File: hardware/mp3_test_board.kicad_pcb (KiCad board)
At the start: 4 copper layers, 99.5 x 56 mm, 224 parts, among them J1 TF01-A, J2 PJ-322, P1 WF24LTYAJDNN0#, P2 USB-TYPE-C-018, Q1 2N7002K, SW1 K2-1156SP-F5SW-05, SW2 K2-1156SP-F5SW-05, SW3 K2-1156SP-F5SW-05, SW4 K2-1156SP-F5SW-05, SW5 K2-1156SP-F5SW-05, SW6 GT-TC054A-H035-L1, SW7 GT-TC054A-H035-L1, SW8 GT-TC054A-H035-L1, U1 F133, U10 SGM6603-ADJYN6G, U11 SGM3204, U2 USBLC6-2SC6, U3 MX25L25645GM2I-08G, U4 PCM1795, U5 LM4562, U6 LM4562, U7 OPA1656, U8 OPA1656, U9 AXP2101, Y1 12.88727, Y2 26МHz

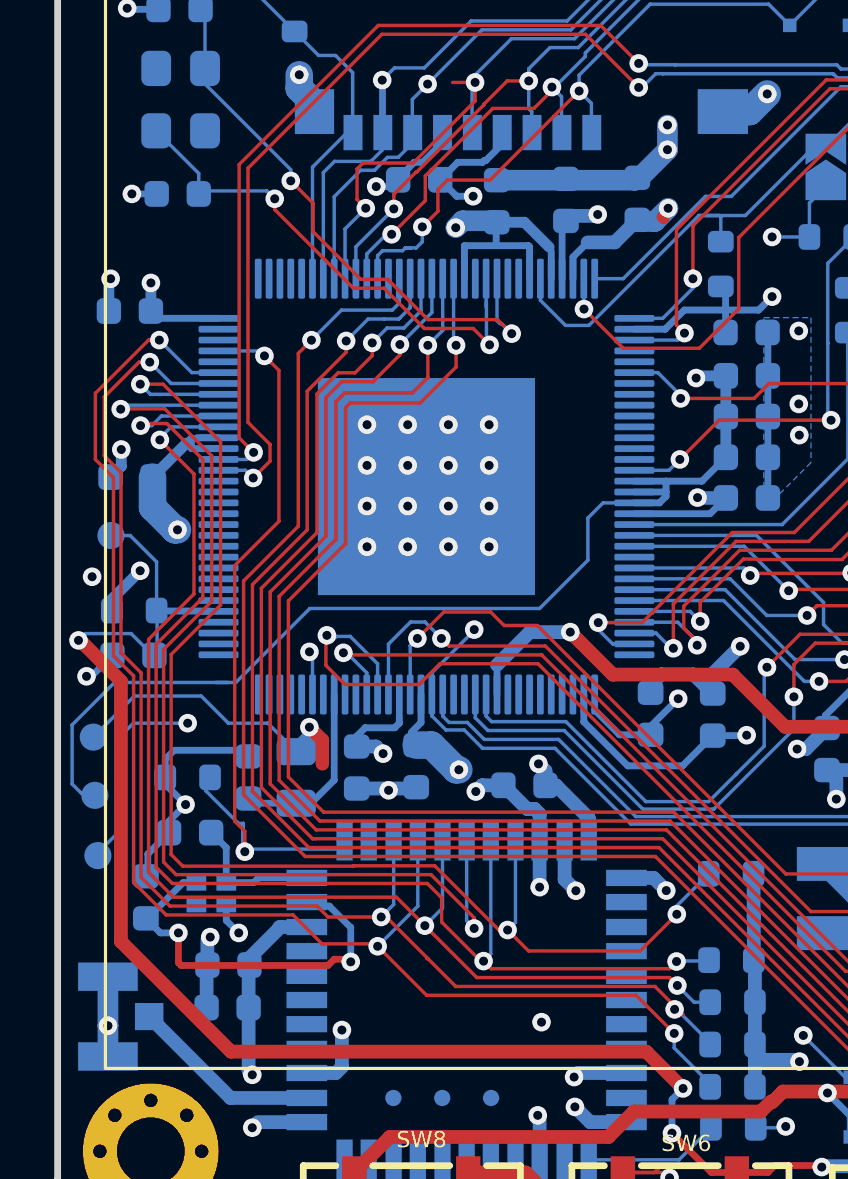
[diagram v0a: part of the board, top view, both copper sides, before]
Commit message: some fixes
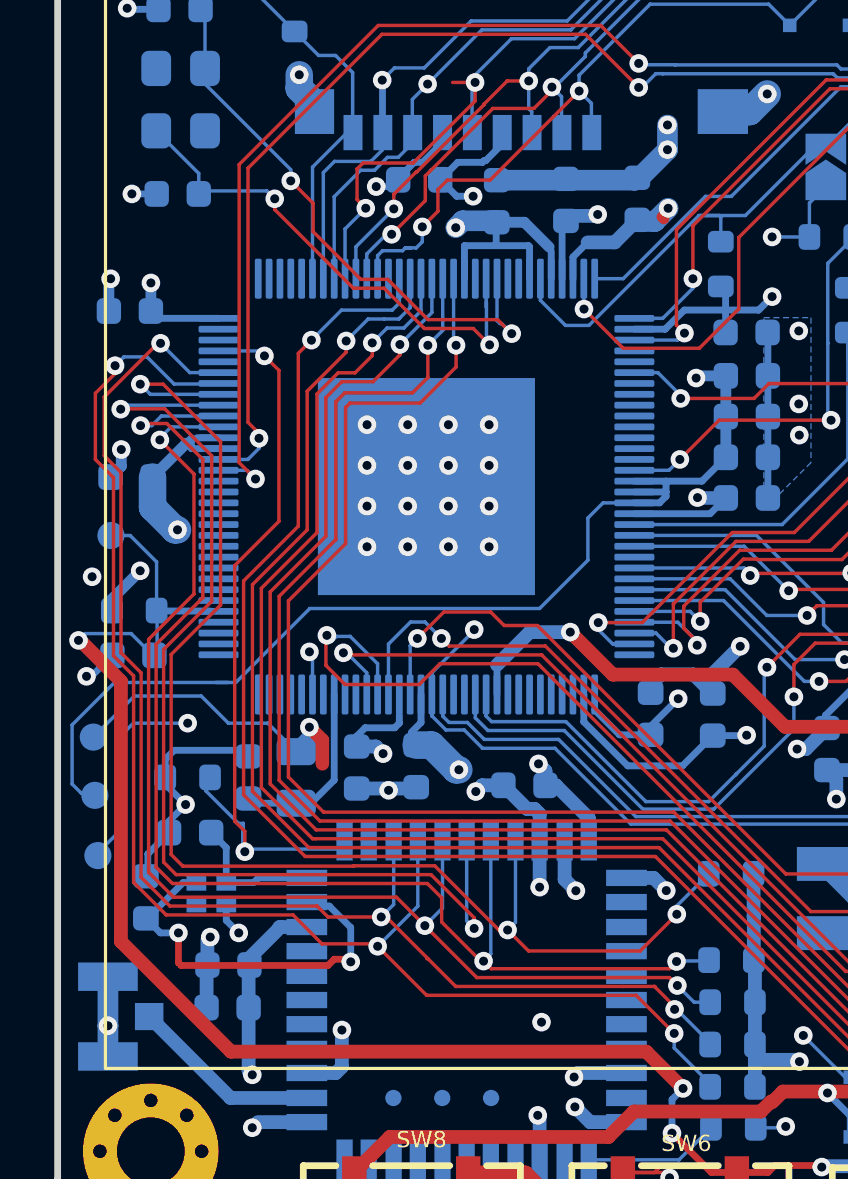
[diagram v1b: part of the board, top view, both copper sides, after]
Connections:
- U1 pad 114: /SOC/USB_DP -> /SOC/USB_DM
- U1 pad 115: /SOC/USB_DM -> /SOC/USB_DP
- U1 pad 122: /SOC/WIFI_SDIO_D2 -> /SOC/WIFI_SDIO_D3
- U1 pad 123: /SOC/WIFI_SDIO_D3 -> /SOC/WIFI_SDIO_D2
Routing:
- net GND: track 394.7 -> 386.3 mm
- net unconnected-(SW3-Pad4): track 0.00 -> 8.35 mm
- net /SOC/USB_DP: track 112.7 -> 111.5 mm
- net /SOC/USB_DM: track 118.9 -> 120.0 mm

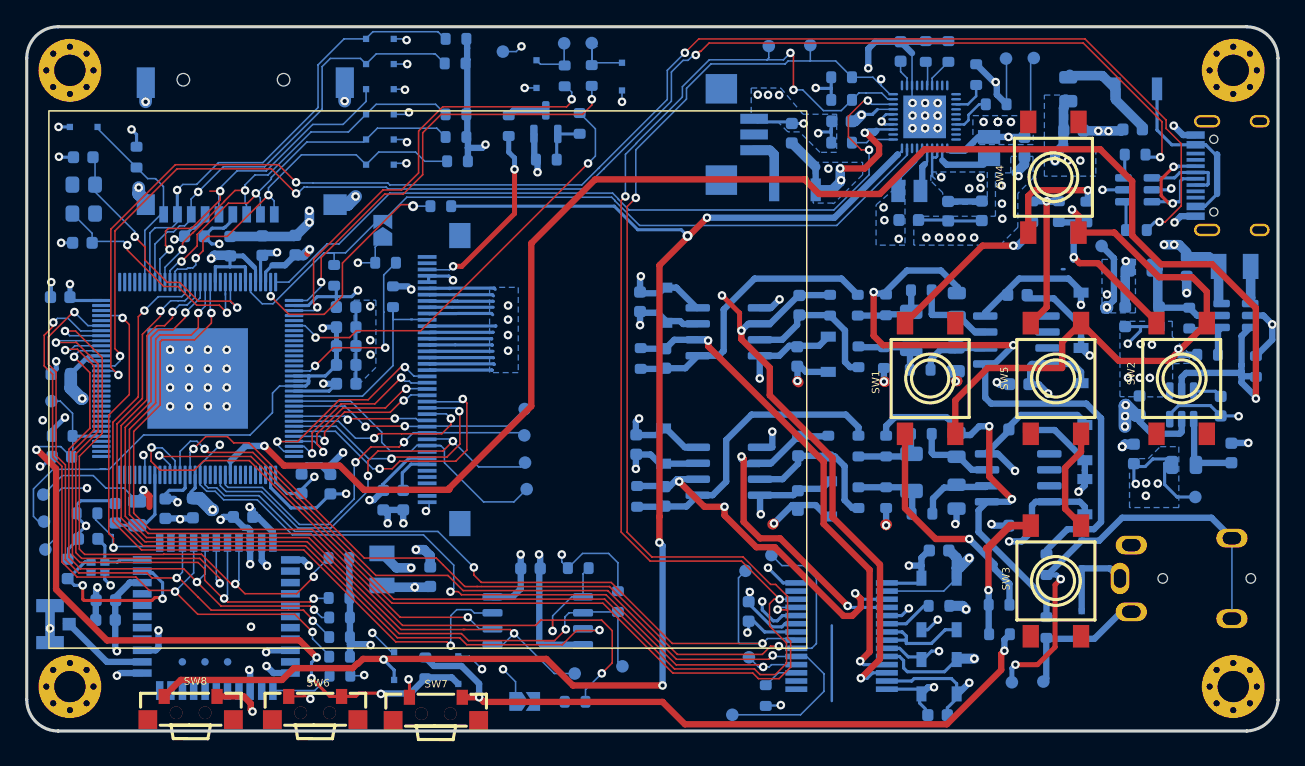
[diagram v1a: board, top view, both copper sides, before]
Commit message: xxx
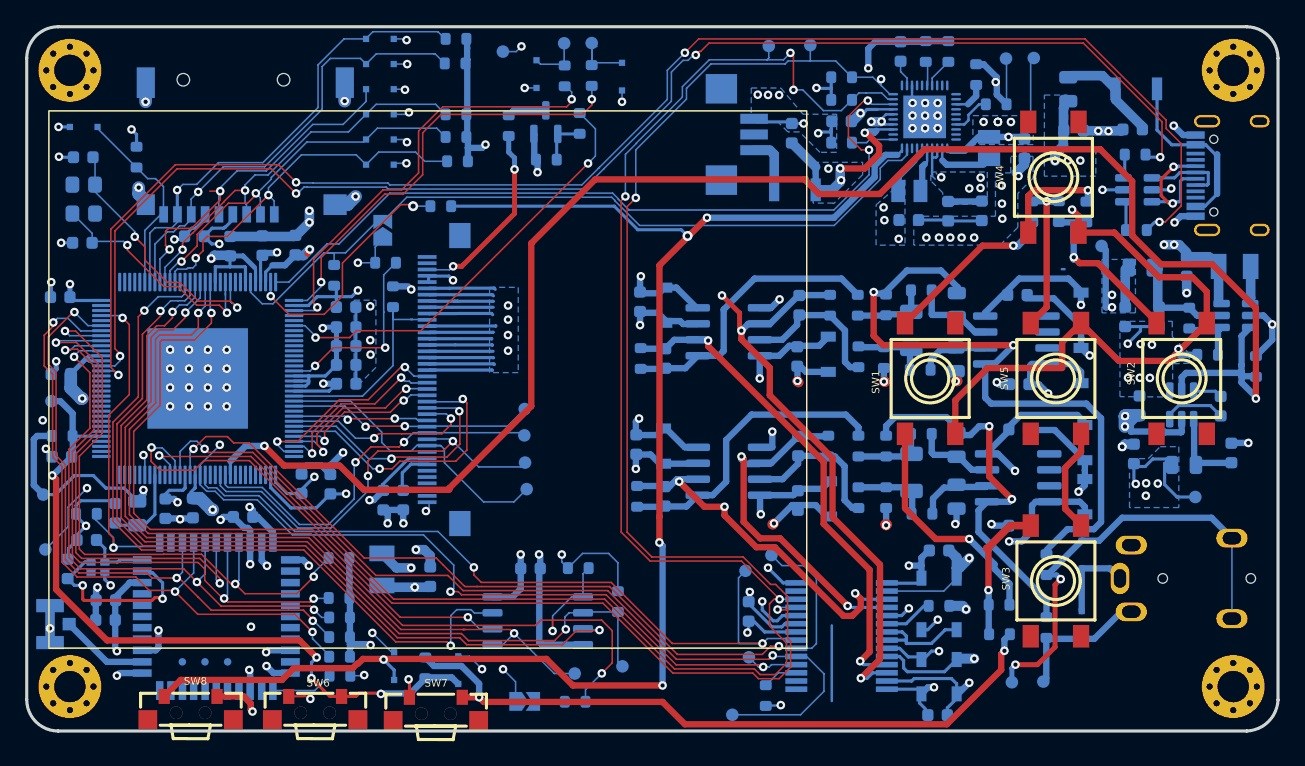
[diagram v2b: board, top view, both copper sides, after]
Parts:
- removed TP7: TestPoint, rlib_misc:TestPoint_Pad_D1.0mm
- C31: value 10u -> 47u
- R6: value 100 -> 50
- moved C77 0.14 mm to (81.2, 84.0)
- moved C64 0.12 mm to (155.8, 52.9)
- moved R64 0.06 mm to (81.2, 82.0)
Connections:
- R5 pad 1: +3V3 -> +1V8A
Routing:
- net +1V8B: track 52.5 -> 23.7 mm
- net unconnected-(SW3-Pad4): track 8.35 -> 0.00 mm
- net +1V8A: track 61.8 -> 66.5 mm
- net GND: track 386.3 -> 390.4 mm
- net /SOC/KEYS: track 60.9 -> 57.3 mm
- net +3V3: track 405.4 -> 403.5 mm, vias 26 -> 25
- net +5VA: track 170.1 -> 168.2 mm, vias 14 -> 12
- net VCC: track 64.4 -> 65.9 mm, vias 8 -> 9
- net Net-(C71-Pad2): track 7.02 -> 5.58 mm, vias 1 -> 0
- net +0V9: track 137.3 -> 136.1 mm
- net -5VA: track 152.7 -> 153.8 mm
- net /SOC/WIFI_REG_ON: track 28.9 -> 27.9 mm
- net /Power/RESET: track 62.1 -> 62.6 mm
